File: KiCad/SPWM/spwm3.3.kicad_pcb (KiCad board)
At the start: 2 copper layers, 70 x 20 mm, 17 parts, among them U1 SMARTPWM V3, U4 24G PAD, U5 24G PAD, U6 24G PAD, U7 24G PAD

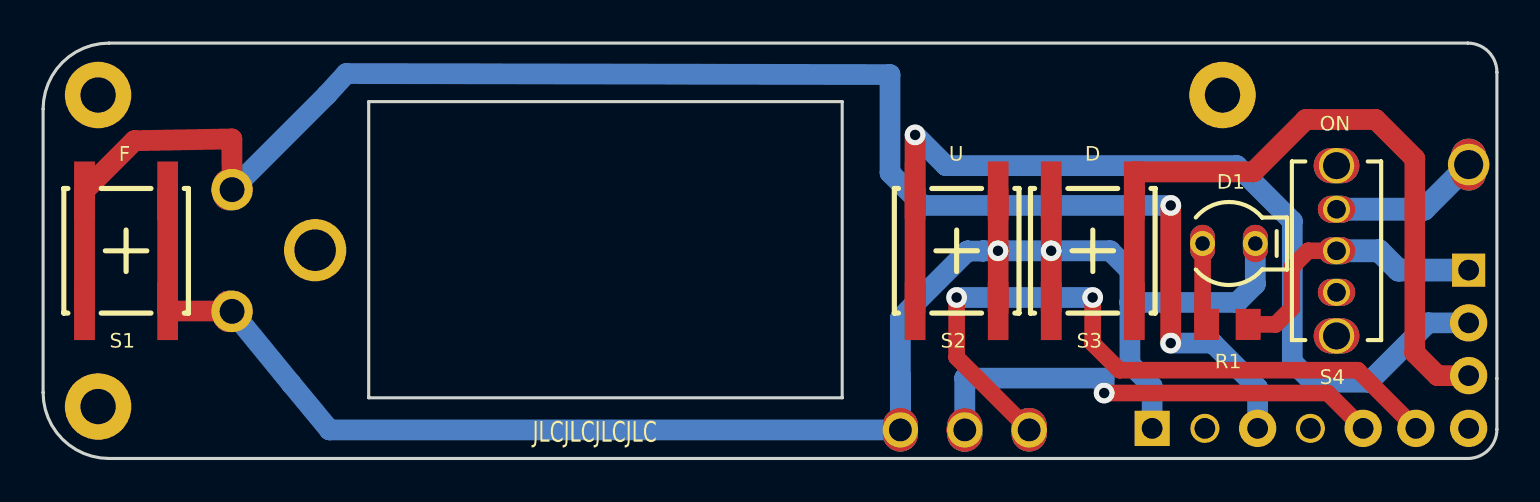
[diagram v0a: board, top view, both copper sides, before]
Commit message: Cleanup and make pretty rendering
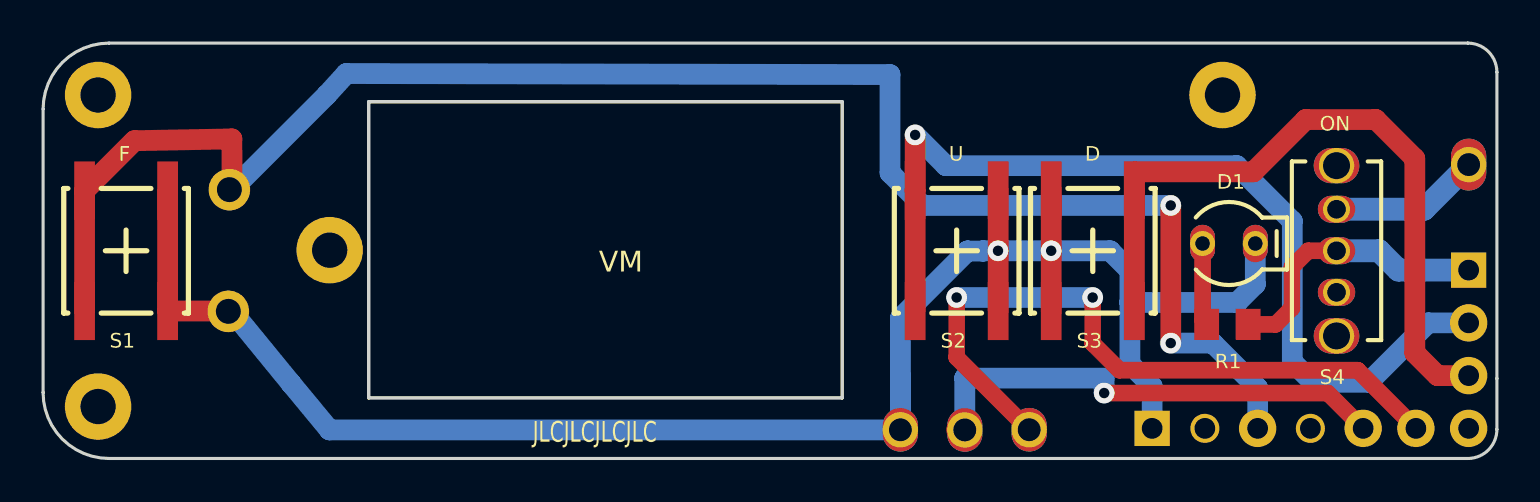
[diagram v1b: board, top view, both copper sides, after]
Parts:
- added VM: VM, spwm3.3:VM, F.Cu at (140.7, 105.1)
- D1: footprint vm-moved:SSL-LX40FT3ID -> spwm3.3:SSL-LX40FT3ID
- Pad1, Pad3, Pad5, Pad6: footprint vm-moved:Pad -> spwm3.3:Pad
- Pad4: footprint vm-moved:Pad_Pad4 -> spwm3.3:Pad_Pad4
- Pad7: footprint vm-moved:Pad_Pad7 -> spwm3.3:Pad_Pad7
- R1: footprint vm-moved:RES_0805edit -> spwm3.3:RES_0805edit
- S2, S3: footprint vm-moved:KSC641JLFS -> spwm3.3:KSC641JLFS
- S4: footprint vm-moved:SS-12D07-VG4NSGAPA -> spwm3.3:SS-12D07-VG4NSGAPA
- U1: footprint vm-moved:SmartPWM_V3 -> spwm3.3:SmartPWM_V3
- U4: footprint vm-moved:24g_pad_U4 -> spwm3.3:24g_pad_U4
- U5, U6, U7: footprint vm-moved:24g_pad_U5 -> spwm3.3:24g_pad_U5
